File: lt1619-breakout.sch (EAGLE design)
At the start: 20 parts

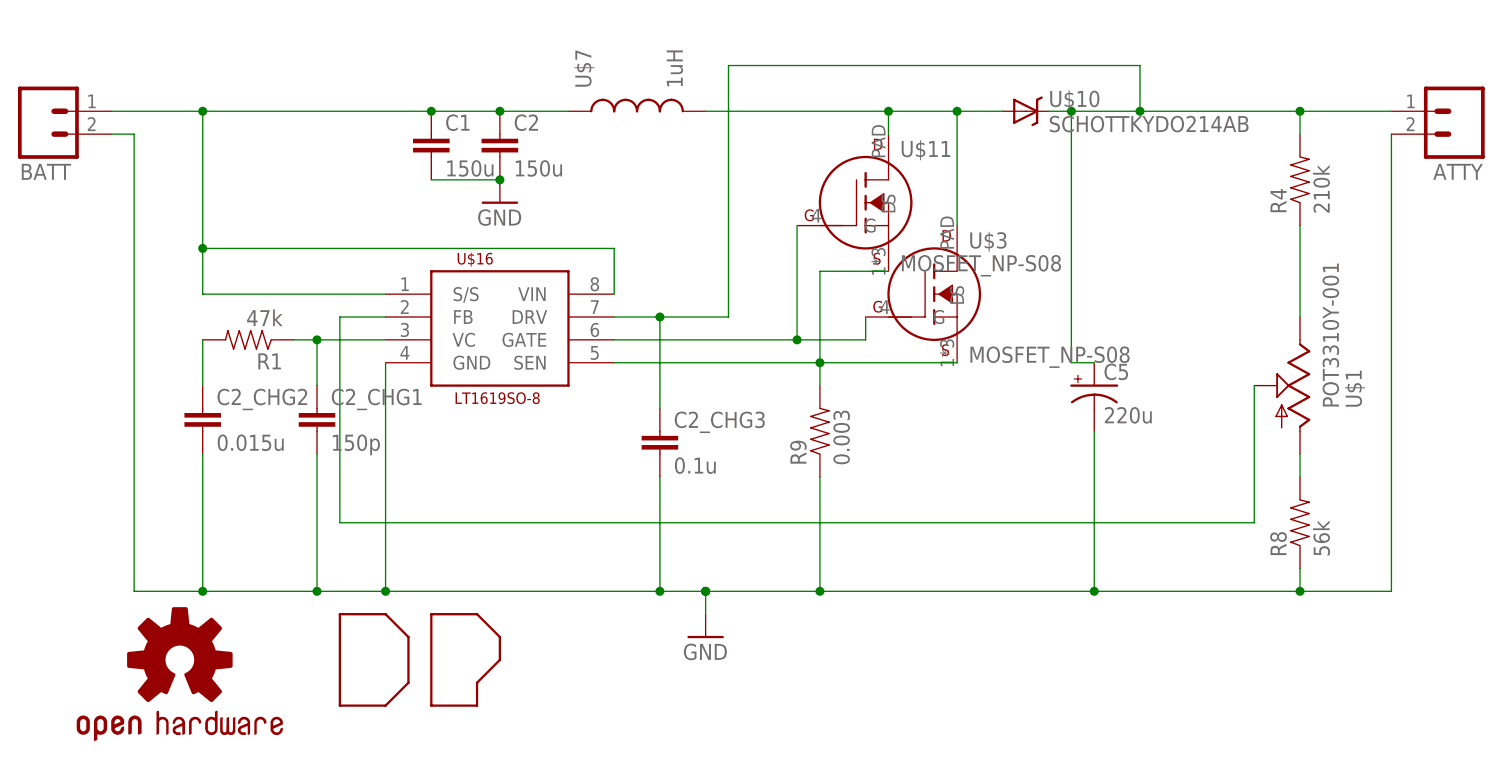
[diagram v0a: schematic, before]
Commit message: schematic cleanup
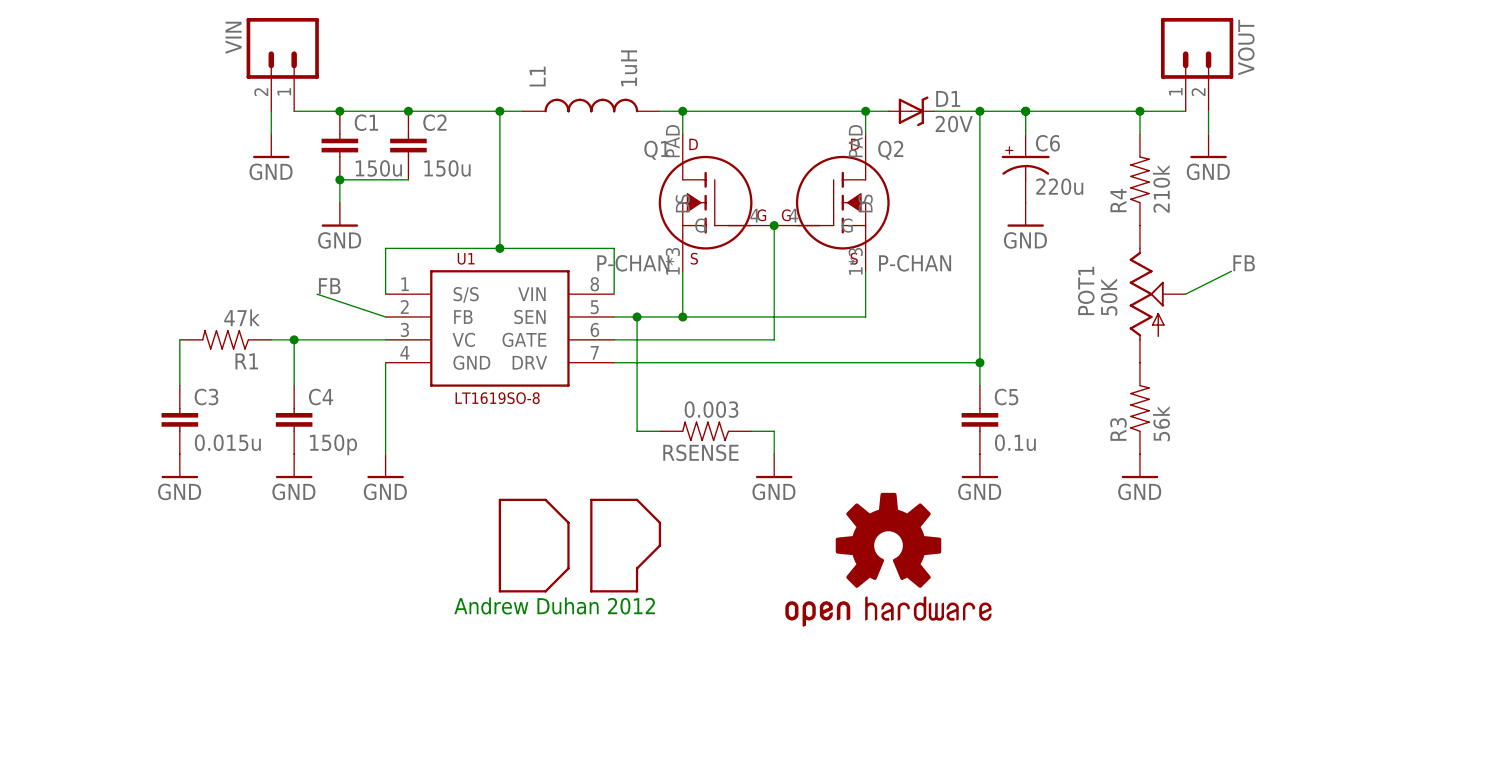
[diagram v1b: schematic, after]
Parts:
- removed ATTY, BATT: (no value), SparkFun-Connectors:M02PTH
- removed C2_CHG1: 150p, SparkFun:CAP0603-CAP
- removed C2_CHG2: 0.015u, SparkFun:CAP0603-CAP
- removed C2_CHG3: 0.1u, SparkFun:CAP0603-CAP
- removed R8: 56k, SparkFun-Passives:RESISTOR0603-RES
- removed R9: 0.003, SparkFun-Passives:RESISTOR1206
- removed U$1: POT3310Y-001, myparts:POT3310Y-001
- removed U$10: SCHOTTKYDO214AB, myparts:SCHOTTKYDO214AB
- removed U$11, U$3: MOSFET_NP-S08, myparts:MOSFET_NP-S08
- removed U$7: 1uH, myparts:INDUCTOR-SMD-MED4
- added C3: 0.015u, SparkFun:CAP0603-CAP
- added C4: 150p, SparkFun:CAP0603-CAP
- added C6: 220u, SparkFun-Passives:CAP_POL7343
- added D1: 20V, myparts:SCHOTTKYDO214AB
- added L1: 1uH, myparts:INDUCTOR-SMD-MED4
- added POT1: 50K, myparts:POT3310Y-001
- added Q1, Q2: P-CHAN, myparts:MOSFET_NP-S08
- added R3: 56k, SparkFun-Passives:RESISTOR0603-RES
- added RSENSE: 0.003, SparkFun-Passives:RESISTOR1206
- added VIN, VOUT: (no value), SparkFun-Connectors:M02PTH
- C5: value 220u -> 0.1u; device SparkFun-Passives:CAP_POL7343 -> SparkFun:CAP0603-CAP
- renumbered U$16 to U1
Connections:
- removed net N$16: U$1.W, U1.FB
- removed net N$3: U$10.A, U$11.D, U$3.D, U$7.2
- removed net N$4: U$11.G, U$3.G, U1.GATE
- removed net N$7: R9.2, U$11.S, U$3.S, U1.SEN
- removed net V_ATTY: ATTY.1, C2_CHG3.1, C5.+, R4.2, U$10.C, U1.DRV
- removed net V_BATT: BATT.1, C1.1, C2.1, U$7.1, U1.S/S, U1.VIN
- new net DRAIN: D1.A, L1.2, Q1.D, Q2.D
- new net FB: POT1.W, U1.FB
- new net GATE: Q1.G, Q2.G, U1.GATE
- new net SOURCE: Q1.S, Q2.S, RSENSE.2, U1.SEN
- new net VBATT: C1.1, C2.1, L1.1, U1.S/S, U1.VIN, VIN.1
- new net VOUT: C5.1, C6.+, D1.C, R4.2, U1.DRV, VOUT.1
- net GND: now also C3.2, C4.2, C5.2, C6.-, R3.1, RSENSE.1, VIN.2, VOUT.2; no longer ATTY.2, BATT.2, C2_CHG1.2, C2_CHG2.2, C2_CHG3.2, C5.-, R8.1, R9.1
- net N$1: now also C3.1; no longer C2_CHG2.1
- net N$2: now also POT1.B; no longer U$1.B
- net N$5: now also C4.1; no longer C2_CHG1.1
- net N$8: now also POT1.A, R3.2; no longer R8.2, U$1.A
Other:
- note added: "Andrew Duhan 2012"
- moved on the sheet: C1, C2, R1, R4
